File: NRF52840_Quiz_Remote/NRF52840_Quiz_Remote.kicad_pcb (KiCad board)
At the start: 2 copper layers, 66 x 173 mm, 28 parts, among them J1 NRF_LEFT, J2 NRF_RIGHT, SW1 ANSWER_A, SW2 ANSWER_B, SW3 ANSWER_C, SW4 ANSWER_D, SW5 SUBMIT, SW6 POWER, SW7 RESET

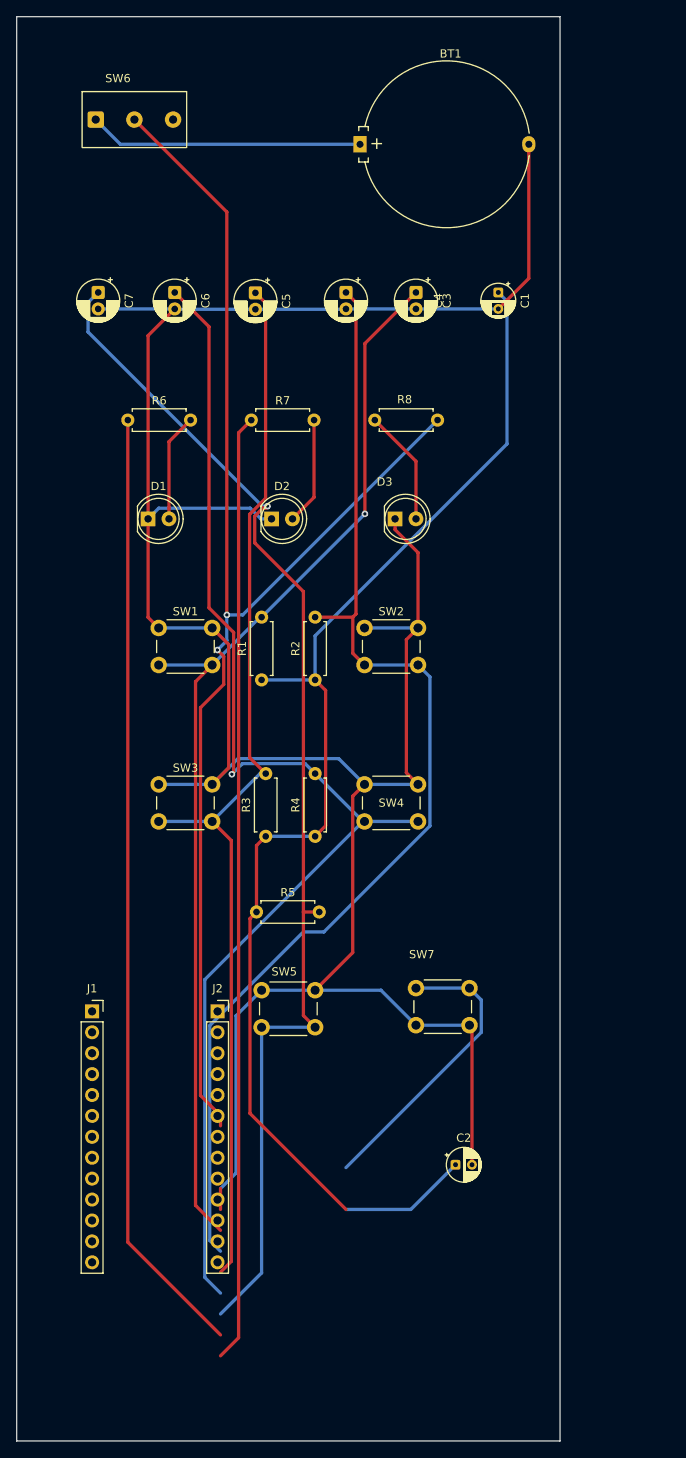
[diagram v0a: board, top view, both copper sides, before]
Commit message: web
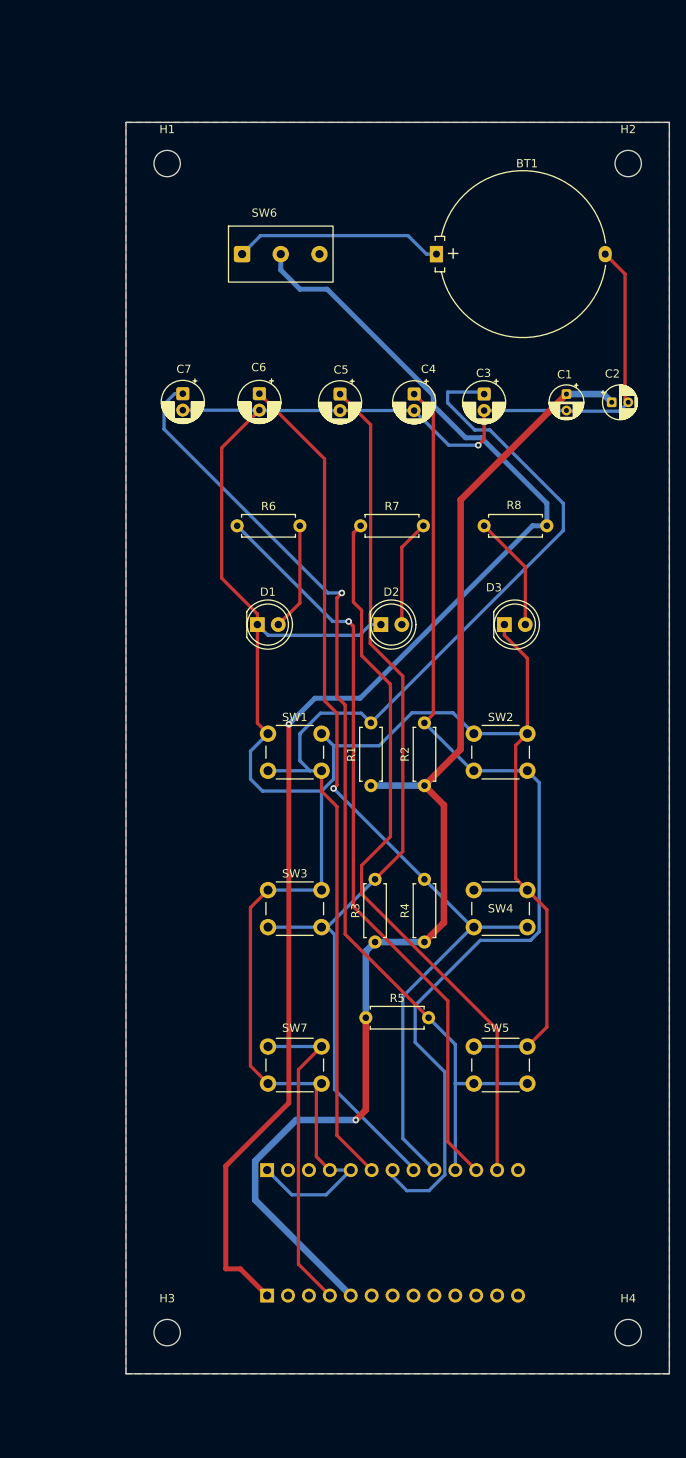
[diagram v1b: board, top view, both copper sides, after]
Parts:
- added H1: MountingHole_3.2mm_M3, MountingHole:MountingHole_3.2mm_M3, F.Cu at (75.4, 36.7)
- added H2: MountingHole_3.2mm_M3, MountingHole:MountingHole_3.2mm_M3, F.Cu at (131.4, 36.7)
- added H3: MountingHole_3.2mm_M3, MountingHole:MountingHole_3.2mm_M3, F.Cu at (75.4, 178.7)
- added H4: MountingHole_3.2mm_M3, MountingHole:MountingHole_3.2mm_M3, F.Cu at (131.4, 178.7)
- J1, J2: moved to B.Cu
- moved C2 94.5 mm to (129.4, 65.7)
- moved J2 35.0 mm to (87.5, 174.2), turned to -90 degrees
- moved J1 28.7 mm to (87.5, 159.0), turned to -90 degrees
- moved SW5 26.7 mm to (112.6, 144.0)
- moved SW6 24.1 mm to (89.2, 47.7)
- moved SW7 19.3 mm to (87.6, 144.0)
- moved R3 18.5 mm to (100.6, 131.3)
- moved R4 18.5 mm to (106.6, 131.3)
- moved R1 18.5 mm to (100.1, 112.3)
- moved R2 18.5 mm to (106.6, 112.3)
- moved R5 18.5 mm to (99.5, 140.5)
- moved D1 18.5 mm to (86.3, 92.7)
- moved D2 18.5 mm to (101.3, 92.7)
- moved D3 18.5 mm to (116.3, 92.7)
- moved R6 18.5 mm to (83.9, 80.7)
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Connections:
- J1 pad 1: /B+ -> GND
- J2 pad 1: /B- -> /B+
- J2 pad 3: Net-(J2-Pin_3) -> GND
- SW7 pad 1: Net-(J2-Pin_3) -> /RST
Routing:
- net /RST: track 0.00 -> 39.5 mm
- net /BTN_D: track 153.7 -> 117.1 mm
- net Net-(J2-Pin_3): track 35.7 -> 0.00 mm
- net /BTN_SUB: track 148.4 -> 120.7 mm
- net /LED_SENT: track 115.2 -> 88.8 mm
- net /LED_CONNECT: track 115.8 -> 91.4 mm, vias 0 -> 1
- net /BTN_C: track 132.2 -> 112.8 mm
- net /BTN_B: track 142.5 -> 125.9 mm
- net Net-(BT1-+): track 33.3 -> 25.5 mm
- net GND: track 329.5 -> 334.4 mm, vias 0 -> 1
- net /VCC: track 156.2 -> 152.1 mm, vias 0 -> 1
- net /B+: track 165.2 -> 166.5 mm, vias 2 -> 1
- net /BTN_A: track 132.9 -> 134.0 mm, vias 1 -> 0
- added copper zone on B.Cu, net GND
- added copper zone on F.Cu, net GND
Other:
- board size 66 x 173 mm -> 66 x 152 mm
